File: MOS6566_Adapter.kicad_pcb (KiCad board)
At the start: 2 copper layers, 35.2 x 77.2 mm, 14 parts, among them U1 MOS6566, U2 MOS6567/MOS8562, U3 74HCT04, U4 74HCT245, U5 74HCT573, U6 74HCT573

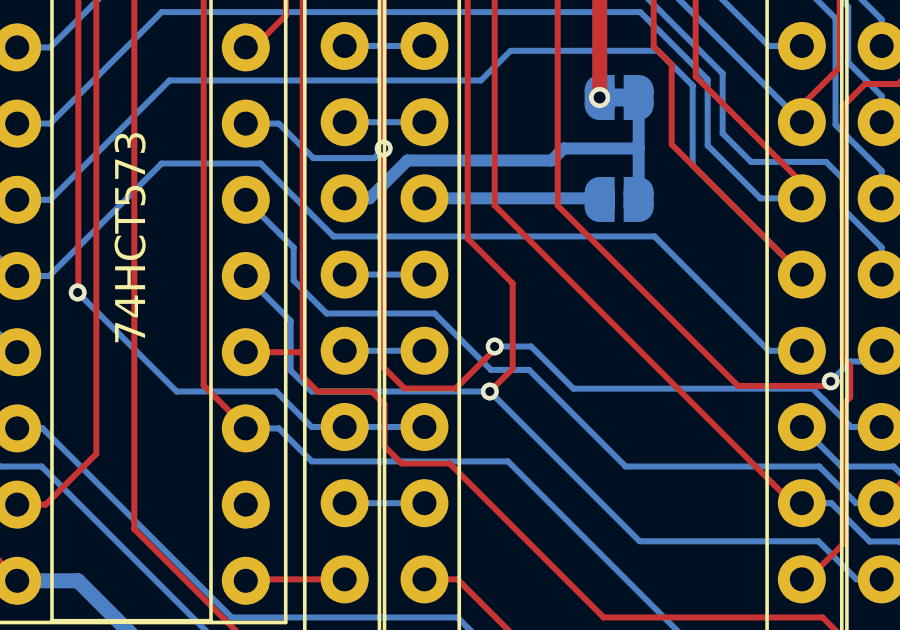
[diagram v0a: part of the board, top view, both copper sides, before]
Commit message: Minor cosmetics
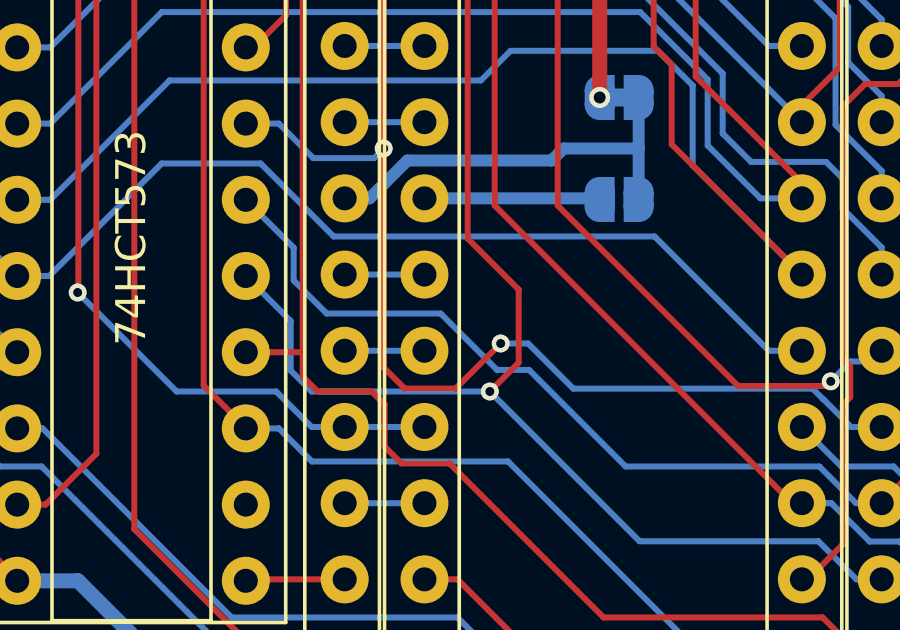
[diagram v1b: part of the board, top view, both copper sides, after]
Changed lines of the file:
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@@
+	)
+	(segment
+		(start 121.3075 39.1517)
+		(end 121.3075 38.05)
+		(width 0.2)
+		(layer "F.Cu")
+		(net 11)
+	)
+	(segment
+		(start 121.8 88.4)
+		(end 120.1 86.7)
+		(width 0.2)
+		(layer "F.Cu")
+		(net 11)
+	)
+	(segment
+		(start 121.8 90.8385)
+		(end 121.8 88.4)
+		(width 0.2)
+		(layer "F.Cu")
+		(net 11)
+	)
+	(segment
+		(start 120.1 40.3592)
+		(end 121.3075 39.1517)
+		(width 0.2)
+		(layer "F.Cu")
+		(net 11)
 	)
 	(segment
@@
 	)
 	(segment
-		(start 120.1 40.3592)
-		(end 121.3075 39.1517)
-		(width 0.2)
-		(layer "F.Cu")
-		(net 11)
-	)
-	(segment
-		(start 121.6 91.0385)
-		(end 121.6 88.2)
-		(width 0.2)
-		(layer "F.Cu")
-		(net 11)
-	)
-	(segment
-		(start 121.6 88.2)
-		(end 120.1 86.7)
-		(width 0.2)
-		(layer "F.Cu")
-		(net 11)
-	)
-	(segment
 		(start 120.8385 91.8)
-		(end 121.6 91.0385)
-		(width 0.2)
-		(layer "F.Cu")
-		(net 11)
-	)
-	(segment
-		(start 121.3075 39.1517)
-		(end 121.3075 38.05)
+		(end 121.8 90.8385)
 		(width 0.2)
 		(layer "F.Cu")
@@
 	)
 	(segment
+		(start 114.3 88.1)
+		(end 115.4 89.2)
+		(width 0.2)
+		(layer "B.Cu")
+		(net 31)
+	)
+	(segment
+		(start 133.0445 95.522)
+		(end 133.9 95.522)
+		(width 0.2)
+		(layer "B.Cu")
+		(net 31)
+	)
+	(segment
+		(start 131.8225 94.3)
+		(end 133.0445 95.522)
+		(width 0.2)
+		(layer "B.Cu")
+		(net 31)
+	)
+	(segment
+		(start 119.1986 89.2)
+		(end 121.0782 91.0796)
+		(width 0.2)
+		(layer "B.Cu")
+		(net 31)
+	)
+	(segment
+		(start 115.4 89.2)
+		(end 119.1986 89.2)
+		(width 0.2)
+		(layer "B.Cu")
+		(net 31)
+	)
+	(segment
 		(start 125.3656 94.3)
 		(end 131.8225 94.3)
@@
 	)
 	(segment
+		(start 121.0782 91.0796)
+		(end 122.1452 91.0796)
+		(width 0.2)
+		(layer "B.Cu")
+		(net 31)
+	)
+	(segment
 		(start 112.704 85.41)
 		(end 114.3 87.006)
@@
 	)
 	(segment
-		(start 131.8225 94.3)
-		(end 133.0445 95.522)
-		(width 0.2)
-		(layer "B.Cu")
-		(net 31)
-	)
-	(segment
-		(start 118.9972 89.2)
-		(end 120.8768 91.0796)
-		(width 0.2)
-		(layer "B.Cu")
-		(net 31)
-	)
-	(segment
-		(start 133.0445 95.522)
-		(end 133.9 95.522)
-		(width 0.2)
-		(layer "B.Cu")
-		(net 31)
-	)
-	(segment
-		(start 114.3 88.1)
-		(end 115.4 89.2)
+		(start 114.3 87.006)
+		(end 114.3 88.1)
 		(width 0.2)
 		(layer "B.Cu")
@@
 	)
 	(segment
-		(start 115.4 89.2)
-		(end 118.9972 89.2)
-		(width 0.2)
-		(layer "B.Cu")
-		(net 31)
-	)
-	(segment
-		(start 114.3 87.006)
-		(end 114.3 88.1)
-		(width 0.2)
-		(layer "B.Cu")
-		(net 31)
-	)
-	(segment
-		(start 120.8768 91.0796)
-		(end 122.1452 91.0796)
-		(width 0.2)
-		(layer "B.Cu")
-		(net 31)
-	)
-	(segment
 		(start 118.66 80.282)
 		(end 116 80.282)
@@
 	)
 	(segment
+		(start 117.3 91)
+		(end 117.3 83.7)
+		(width 0.2)
+		(layer "F.Cu")
+		(net 33)
+	)
+	(segment
 		(start 118 91.7)
 		(end 117.3 91)
@@
 	)
 	(segment
-		(start 117.3 91)
-		(end 117.3 83.7)
+		(start 121.2 90.2)
+		(end 119.7 91.7)
+		(width 0.2)
+		(layer "F.Cu")
+		(net 33)
+	)
+	(segment
+		(start 119.33035 50.33035)
+		(end 117.3 52.3607)
 		(width 0.2)
 		(layer "F.Cu")
@@
 		(start 119.7 91.7)
 		(end 118 91.7)
-		(width 0.2)
-		(layer "F.Cu")
-		(net 33)
-	)
-	(segment
-		(start 121 90.3)
-		(end 121 90.4)
-		(width 0.2)
-		(layer "F.Cu")
-		(net 33)
-	)
-	(segment
-		(start 119.33035 50.33035)
-		(end 117.3 52.3607)
-		(width 0.2)
-		(layer "F.Cu")
-		(net 33)
-	)
-	(segment
-		(start 121 90.4)
-		(end 119.7 91.7)
 		(width 0.2)
 		(layer "F.Cu")
@@
 	)
 	(via
-		(at 121 90.3)
+		(at 121.2 90.2)
 		(size 0.6)
 		(drill 0.3)
@@
 	)
 	(segment
+		(start 131.954471 92.0613)
+		(end 131.9613 92.0613)
+		(width 0.2)
+		(layer "B.Cu")
+		(net 33)
+	)
+	(segment
+		(start 127.7 39.3625)
+		(end 126.3875 38.05)
+		(width 0.2)
+		(layer "B.Cu")
+		(net 33)
+	)
+	(segment
+		(start 127.7 41.9)
+		(end 127.7 39.3625)
+		(width 0.2)
+		(layer "B.Cu")
+		(net 33)
+	)
+	(segment
+		(start 124.2 42.7)
+		(end 126.9 42.7)
+		(width 0.2)
+		(layer "B.Cu")
+		(net 33)
+	)
+	(segment
+		(start 114.9557 84.02)
+		(end 113.8057 82.87)
+		(width 0.2)
+		(layer "B.Cu")
+		(net 33)
+	)
+	(segment
+		(start 131.9613 92.0613)
+		(end 132.882 92.982)
+		(width 0.2)
+		(layer "B.Cu")
+		(net 33)
+	)
+	(segment
+		(start 117.3 83.7)
+		(end 116.98 84.02)
+		(width 0.2)
+		(layer "B.Cu")
+		(net 33)
+	)
+	(segment
+		(start 123.6213 91.7048)
+		(end 131.603 91.7048)
+		(width 0.2)
+		(layer "B.Cu")
+		(net 33)
+	)
+	(segment
+		(start 131.603 91.7048)
+		(end 131.603 91.709829)
+		(width 0.2)
+		(layer "B.Cu")
+		(net 33)
+	)
+	(segment
+		(start 116.98 84.02)
+		(end 114.9557 84.02)
+		(width 0.2)
+		(layer "B.Cu")
+		(net 33)
+	)
+	(segment
 		(start 132.882 92.982)
 		(end 133.9 92.982)
@@
 	)
 	(segment
-		(start 127.7 39.3625)
-		(end 126.3875 38.05)
+		(start 113.8057 82.87)
+		(end 112.704 82.87)
+		(width 0.2)
+		(layer "B.Cu")
+		(net 33)
+	)
+	(segment
+		(start 120.0415 49.6192)
+		(end 120.0415 46.8585)
+		(width 0.2)
+		(layer "B.Cu")
+		(net 33)
+	)
+	(segment
+		(start 121.2 90.2)
+		(end 122.1165 90.2)
+		(width 0.2)
+		(layer "B.Cu")
+		(net 33)
+	)
+	(segment
+		(start 122.1165 90.2)
+		(end 123.6213 91.7048)
+		(width 0.2)
+		(layer "B.Cu")
+		(net 33)
+	)
+	(segment
+		(start 126.9 42.7)
+		(end 127.7 41.9)
+		(width 0.2)
+		(layer "B.Cu")
+		(net 33)
+	)
+	(segment
+		(start 119.33035 50.33035)
+		(end 120.0415 49.6192)
 		(width 0.2)
 		(layer "B.Cu")
@@
 		(width 0.2)
 		(layer "B.Cu")
-		(net 33)
-	)
-	(segment
-		(start 127.7 41.9)
-		(end 127.7 39.3625)
-		(width 0.2)
-		(layer "B.Cu")
-		(net 33)
-	)
-	(segment
-		(start 124.2 42.7)
-		(end 126.9 42.7)
-		(width 0.2)
-		(layer "B.Cu")
-		(net 33)
-	)
-	(segment
-		(start 114.9557 84.02)
-		(end 113.8057 82.87)
-		(width 0.2)
-		(layer "B.Cu")
-		(net 33)
-	)
-	(segment
-		(start 131.9613 92.0613)
-		(end 132.882 92.982)
-		(width 0.2)
-		(layer "B.Cu")
-		(net 33)
-	)
-	(segment
-		(start 117.3 83.7)
-		(end 116.98 84.02)
-		(width 0.2)
-		(layer "B.Cu")
-		(net 33)
-	)
-	(segment
-		(start 131.603 91.7048)
-		(end 131.603 91.709829)
-		(width 0.2)
-		(layer "B.Cu")
-		(net 33)
-	)
-	(segment
-		(start 123.6213 91.7048)
-		(end 131.603 91.7048)
-		(width 0.2)
-		(layer "B.Cu")
-		(net 33)
-	)
-	(segment
-		(start 116.98 84.02)
-		(end 114.9557 84.02)
-		(width 0.2)
-		(layer "B.Cu")
-		(net 33)
-	)
-	(segment
-		(start 113.8057 82.87)
-		(end 112.704 82.87)
-		(width 0.2)
-		(layer "B.Cu")
-		(net 33)
-	)
-	(segment
-		(start 120.0415 49.6192)
-		(end 120.0415 46.8585)
-		(width 0.2)
-		(layer "B.Cu")
-		(net 33)
-	)
-	(segment
-		(start 126.9 42.7)
-		(end 127.7 41.9)
-		(width 0.2)
-		(layer "B.Cu")
-		(net 33)
-	)
-	(segment
-		(start 119.33035 50.33035)
-		(end 120.0415 49.6192)
-		(width 0.2)
-		(layer "B.Cu")
-		(net 33)
-	)
-	(segment
-		(start 121 90.3)
-		(end 122.2165 90.3)
-		(width 0.2)
-		(layer "B.Cu")
-		(net 33)
-	)
-	(segment
-		(start 122.2165 90.3)
-		(end 123.6213 91.7048)
-		(width 0.2)
-		(layer "B.Cu")
-		(net 33)
-	)
-	(segment
-		(start 131.954471 92.0613)
-		(end 131.9613 92.0613)
-		(width 0.2)
-		(layer "B.Cu")
